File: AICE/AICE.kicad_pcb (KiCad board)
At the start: 2 copper layers, 100 x 115 mm, 151 parts, among them J1 Conn_02x10_Odd_Even, J2 Conn_02x10_Odd_Even, J3 Conn_01x03, J4 USB_A, J5 Conn_02x10_Odd_Even, J6 Conn_02x10_Odd_Even, J7 Micro_SD_Card, J8 USB_B_Micro, Q1 S8550, U1 ICE40UP5K-SG48ITR, U10 SMS, U11 DVP_PORT, U12 SMS, U13 ZLDO1117G33TA, U14 ZLDO1117G12TA, U15 ZLDO1117G33TA, U16 ZLDO1117G18TA, U17 XC6206P282MR, U18 XC6206P152MR, U2 ASFLMB-24.00MHZ-LC-T, U3 SMS, U4 W25Q, U5 HX711, U6 Omega2+, U7 SMS, U8 SRF2012, U9 M1&M1W

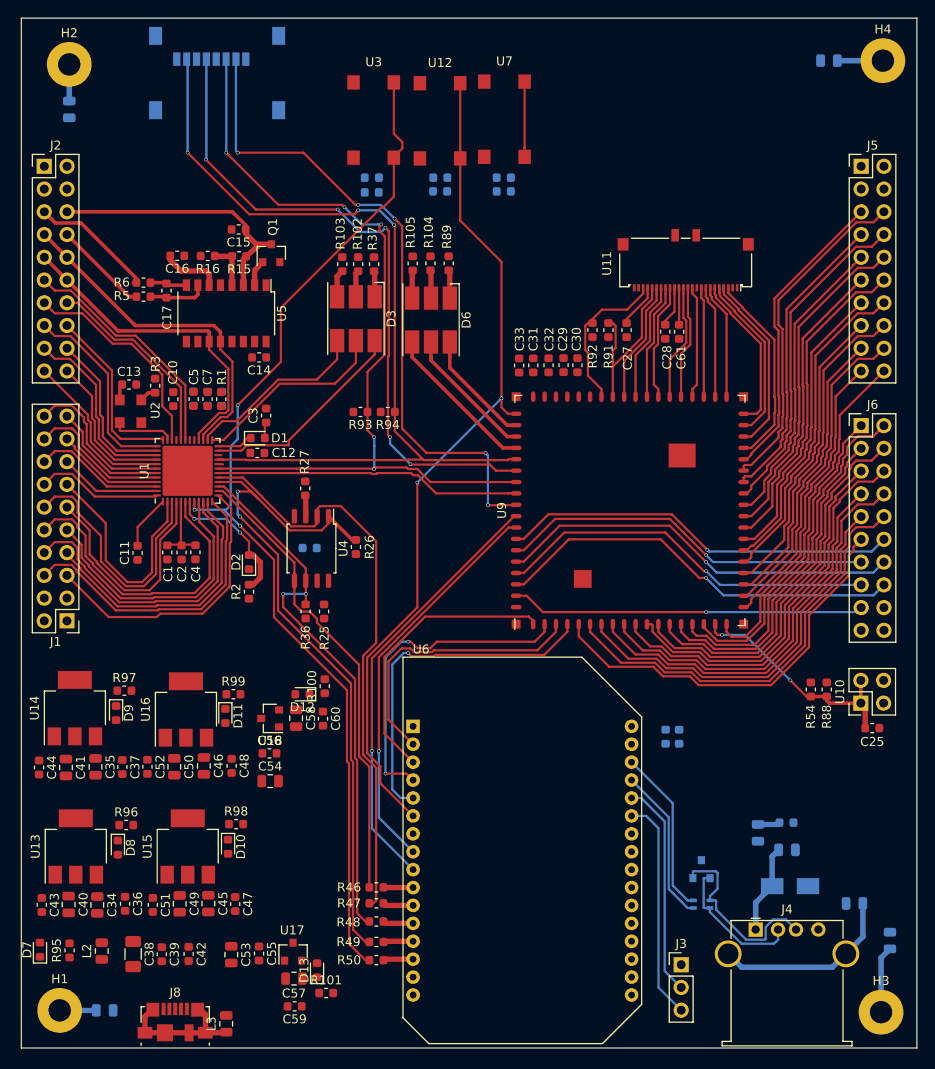
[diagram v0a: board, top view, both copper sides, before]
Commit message: Add files via upload
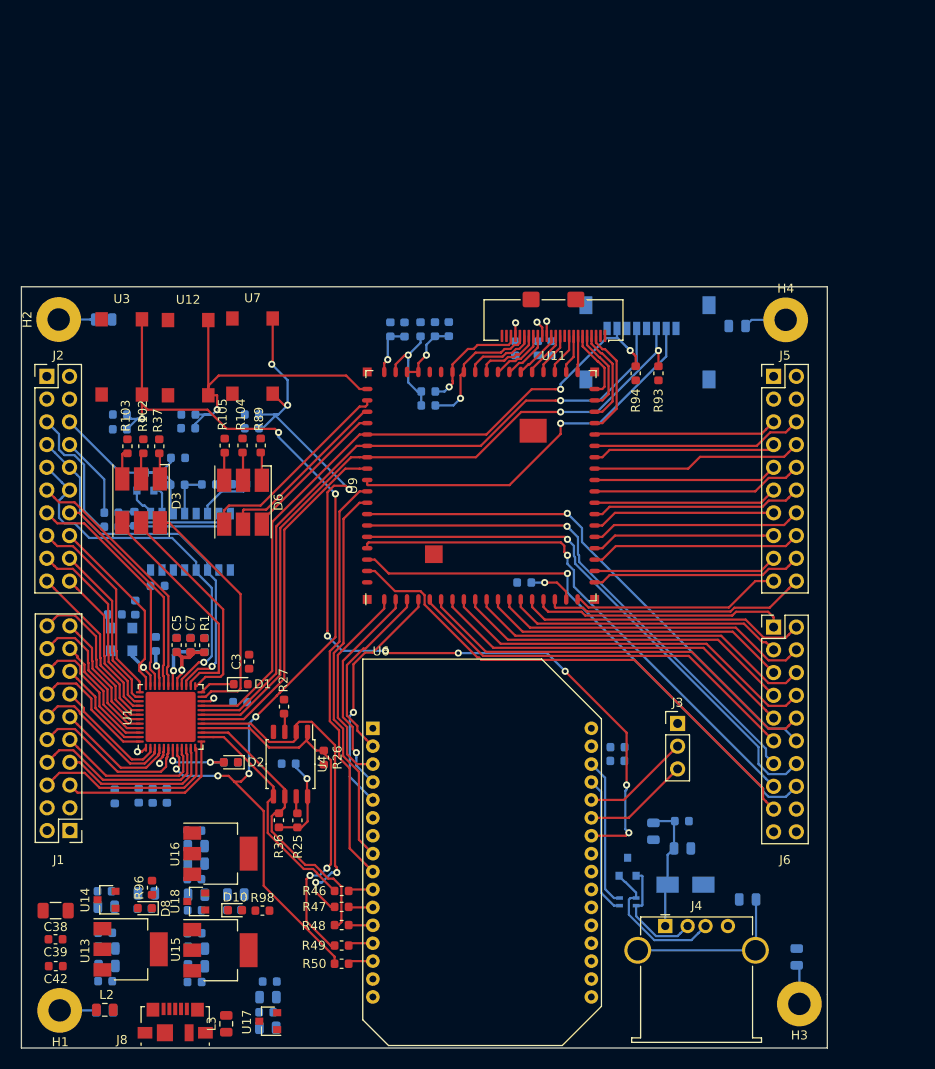
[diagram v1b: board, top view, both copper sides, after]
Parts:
- removed C25: 0.1u, Capacitor_SMD:C_0603_1608Metric
- removed D11: BLU, LED_SMD:LED_0603_1608Metric
- removed D12, D9: GRN, LED_SMD:LED_0603_1608Metric
- removed D13: YLL, LED_SMD:LED_0603_1608Metric
- removed D7: RED, LED_SMD:LED_0603_1608Metric
- removed R100, R101, R95, R97, R99: 2k2, Resistor_SMD:R_0603_1608Metric
- removed R88: 10K, Resistor_SMD:R_0603_1608Metric
- removed U10: SMS, Connector_PinHeader_2.54mm:PinHeader_2x02_P2.54mm_Vertical
- C1, C10, C11, C12, C13, C14, C15, C16, C17, C2, C27, C28, C29, C30, C31, C32, C33, C34, C35, C36, C37, C4, C40, C41, C43, C44, C45, C46, C47, C48, C49, C50, C51, C52, C53, C54, C55, C56, C57, C58, C59, C60, C61, Q1, R15, R16, R2, R3, R5, R54, R6, R91, R92, U2, U5: moved to B.Cu
- U11: footprint Connector_FFC-FPC:Molex_502244-2430_1x24-1MP_P0.5mm_Horizontal -> Connector_FFC-FPC:Molex_502231-2400_1x24-1SH_P0.5mm_Vertical
- U14: value ZLDO1117G12TA -> XC6206P122MR; footprint Package_TO_SOT_SMD:SOT-223 -> Package_TO_SOT_SMD:SOT-23
- moved J7 56.7 mm to (102.9, 70.2)
- moved R90 38.6 mm to (51.6, 79.8)
- moved C19 38.6 mm to (44.0, 78.3)
- moved C24 38.6 mm to (58.7, 78.3)
- moved C26 38.6 mm to (51.7, 78.3)
- moved R4 38.6 mm to (44.0, 79.9)
- moved R53 38.6 mm to (58.7, 79.8), turned to 180 degrees
- moved U12 38.6 mm to (51.6, 71.9)
- moved U3 38.6 mm to (44.2, 71.8)
- moved U7 38.6 mm to (58.8, 71.7)
- moved R54 34.2 mm to (89.2, 97.0), turned to 180 degrees
- moved R93 33.6 mm to (104.1, 73.7), turned to 270 degrees
- moved D3 31.5 mm to (46.4, 87.9)
- moved R103 31.5 mm to (44.8, 81.8)
- moved R37 31.5 mm to (48.4, 81.8)
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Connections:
- J2 pad 10: /iCE40/SDA -> /iCE40/SCK
- J2 pad 12: /iCE40/SCK -> /iCE40/SDA
- J2 pad 7: /iCE40/SDA -> /iCE40/SCK
- J2 pad 9: /iCE40/SCK -> /iCE40/SDA
- U1 pad 27: /iCE40/SDA -> /iCE40/SCK
- U1 pad 28: /iCE40/SCK -> /iCE40/SDA
- U9 pad 56: /sipeedm1w/RGB_R -> /sipeedm1w/RGB_B
- U9 pad 58: /sipeedm1w/RGB_B -> /sipeedm1w/RGB_R
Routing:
- net /omega/RST: track 8.40 -> 103.4 mm, vias 0 -> 9
- net /omega/JTAG4: track 95.0 -> 36.3 mm, vias 2 -> 1
- net /iCE40/OmSPI3: track 79.1 -> 41.8 mm
- net /sipeedm1w/SPI0_CS1: track 74.5 -> 43.7 mm, vias 5 -> 1
- net /iCE40/OmSPI1: track 61.0 -> 32.7 mm, vias 2 -> 0
- net /iCE40/OmSPI0: track 52.1 -> 26.1 mm
- net /iCE40/OmSPI2: track 65.6 -> 39.7 mm, vias 0 -> 2
- net /sipeedm1w/BOOT: track 26.3 -> 5.18 mm, vias 2 -> 1
- net /iCE40/COMM0: track 98.8 -> 78.6 mm, vias 3 -> 2
- net /sipeedm1w/IO33: track 39.5 -> 57.7 mm, vias 1 -> 0
- net /sipeedm1w/IO31: track 42.8 -> 59.3 mm
- net /sipeedm1w/IO29: track 42.0 -> 58.4 mm
- net /iCE40/IO6: track 34.4 -> 18.2 mm
- net /sipeedm1w/IO30: track 45.4 -> 61.6 mm
- net GND_CASE: track 15.3 -> 0.00 mm
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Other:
- board size 100 x 115 mm -> 90 x 85 mm
